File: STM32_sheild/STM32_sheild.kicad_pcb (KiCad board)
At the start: 2 copper layers, 87 x 83.5 mm, 48 parts, among them J1 61612002121503, J2 CN7, J3 CN10, J4 632722100213, J5 691210910002, J6 691210910002, U1 OPA333xxDBV, U2 TPS63031DSK, U3 MCP73831-2-MC, U4 OPA333xxDBV

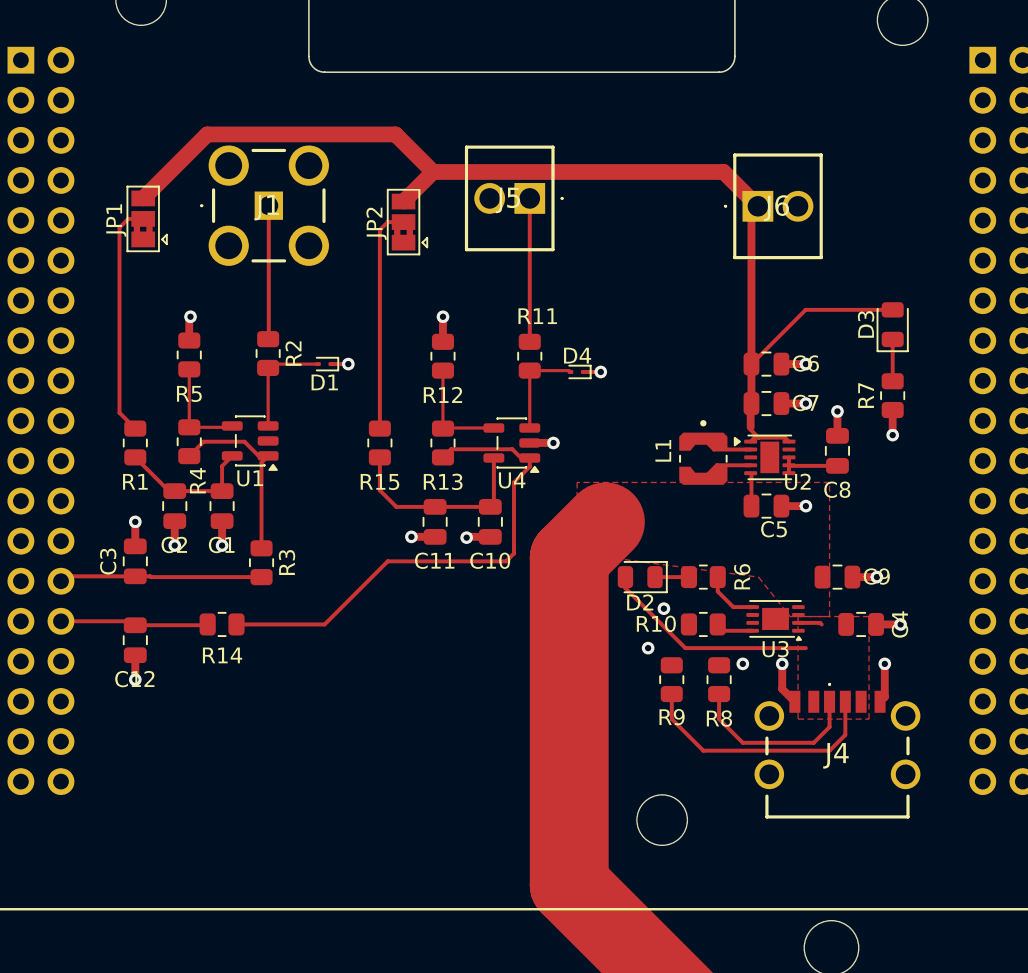
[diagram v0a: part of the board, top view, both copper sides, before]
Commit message: random updates
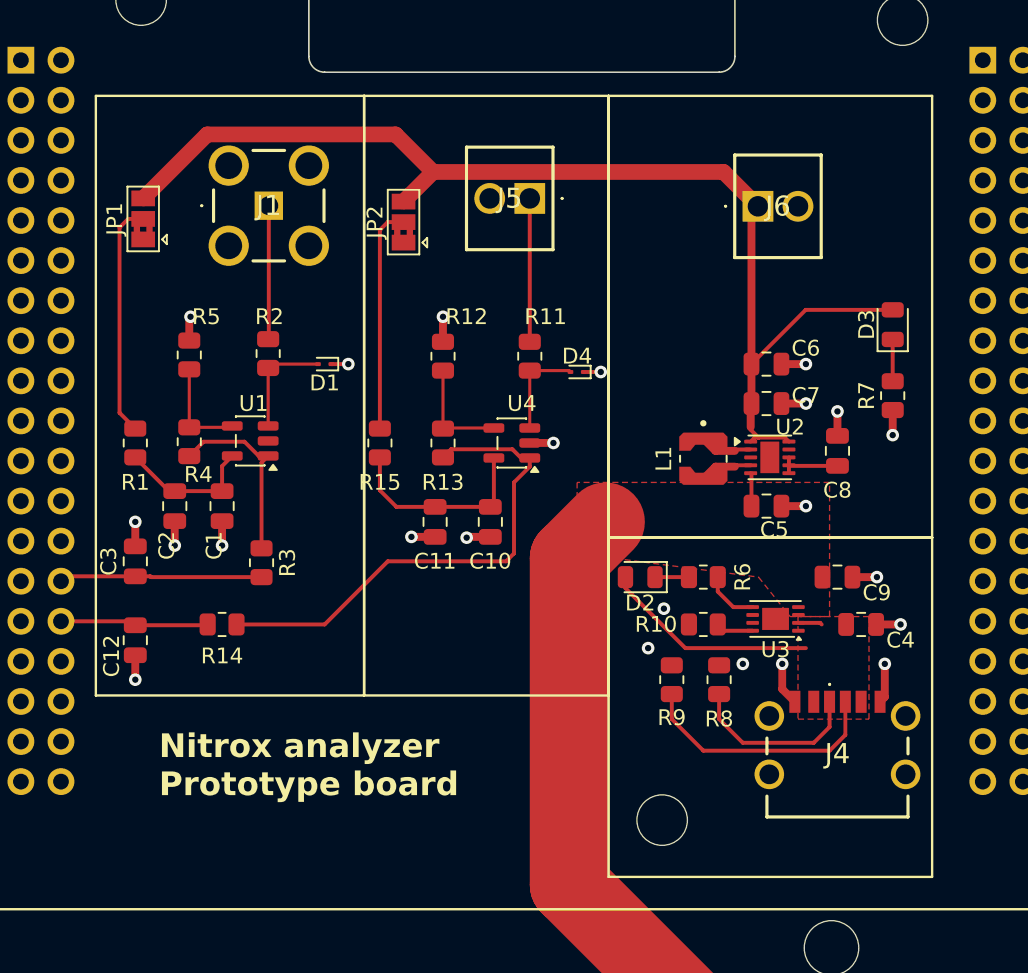
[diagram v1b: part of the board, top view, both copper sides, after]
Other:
- board text added: "Nitrox analyzer Prototype board"
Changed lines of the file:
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@@
 		(tags "resistor")
 		(property "Reference" "R5"
-			(at -2.5 0 180)
+			(at 2.42 1.08 180)
 			(layer "F.SilkS")
 			(effects
@@
 		(tags "WSON NoLead")
 		(property "Reference" "U2"
-			(at 1.7875 1.5875 0)
+			(at 1.2875 -1.9125 0)
 			(layer "F.SilkS")
 			(effects
@@
 		(tags "resistor")
 		(property "Reference" "R2"
-			(at 0 -1.65 90)
+			(at -2.3325 -0.08 180)
 			(layer "F.SilkS")
 			(effects
@@
 		(tags "capacitor")
 		(property "Reference" "C9"
-			(at 2.5 0 180)
+			(at 2.5 1 180)
 			(layer "F.SilkS")
 			(effects
@@
 		)
 		(property "Value" "4.7uF"
-			(at 2 -2 0)
+			(at 0.5 -1.5 0)
 			(layer "F.Fab")
 			(effects
@@
 		(at 148 87.5 -90)
 		(property "Reference" "L1"
-			(at -0.5 2.5 90)
+			(at 0 2.5 270)
 			(layer "F.SilkS")
 			(effects
@@
 		(tags "SOT TO_SOT_SMD")
 		(property "Reference" "U1"
-			(at 0 -2.4 0)
+			(at -0.2175 2.37 0)
 			(layer "F.SilkS")
 			(effects
@@
 		(tags "resistor")
 		(property "Reference" "R12"
-			(at -2.5 0 180)
+			(at 2.5 1.5 180)
 			(layer "F.SilkS")
 			(effects
@@
 		(tags "SOT TO_SOT_SMD")
 		(property "Reference" "U4"
-			(at 0 -2.4 0)
+			(at -0.6375 2.5 0)
 			(layer "F.SilkS")
 			(effects
@@
 		)
 		(property "Value" "OPA333xxDBV"
-			(at -3.1375 2.4 0)
+			(at -4.1375 -2.5 0)
 			(layer "F.Fab")
 			(effects
@@
 		(tags "capacitor")
 		(property "Reference" "C7"
-			(at 2.5 0 0)
+			(at 2.5 -0.5 0)
 			(layer "F.SilkS")
 			(effects
@@
 		)
 		(property "Value" "2.2k"
-			(at -4 0 0)
+			(at -3.5 -1 0)
 			(layer "F.Fab")
 			(effects
@@
 		(tags "capacitor")
 		(property "Reference" "C2"
-			(at 2.5 0 180)
+			(at 2.5 0.5 270)
 			(layer "F.SilkS")
 			(effects
@@
 		)
 		(property "Value" "10uF"
-			(at 0 1.68 90)
+			(at 0.5 1.5 90)
 			(layer "F.Fab")
 			(effects
@@
 		(tags "capacitor")
 		(property "Reference" "C4"
-			(at 2.5 0 90)
+			(at 2.5 1 180)
 			(layer "F.SilkS")
 			(effects
@@
 		(tags "resistor")
 		(property "Reference" "R4"
-			(at 2.5 -0.58 90)
+			(at 2.08 -0.58 180)
 			(layer "F.SilkS")
 			(effects
@@
 		(tags "resistor")
 		(property "Reference" "R11"
-			(at -2.5 -0.5 180)
+			(at -2.5 -1 180)
 			(layer "F.SilkS")
 			(effects
@@
 		(tags "capacitor")
 		(property "Reference" "C12"
-			(at 2.5 0 180)
+			(at 1 1.5 270)
 			(layer "F.SilkS")
 			(effects
@@
 		)
 		(property "Value" "10uF"
-			(at 0 -2.5 90)
+			(at 1 -2 90)
 			(layer "F.Fab")
 			(effects
@@
 		(tags "capacitor")
 		(property "Reference" "C6"
-			(at 2.5 0 180)
+			(at 2.5 -1 180)
 			(layer "F.SilkS")
 			(effects
@@
 		(tags "capacitor")
 		(property "Reference" "C1"
-			(at 2.5 0 180)
+			(at 2.5 0.5 270)
 			(layer "F.SilkS")
 			(effects
@@
 		)
 		(property "Value" "100n"
-			(at 0 -1.5 90)
+			(at 0.5 1.5 90)
 			(layer "F.Fab")
 			(effects
@@
 		)
 	)
+	(gr_rect
+		(start 109.5 64.5)
+		(end 126.5 102.5)
+		(stroke
+			(width 0.15)
+			(type default)
+		)
+		(fill no)
+		(layer "F.SilkS")
+	)
+	(gr_rect
+		(start 126.5 64.5)
+		(end 142 102.5)
+		(stroke
+			(width 0.15)
+			(type default)
+		)
+		(fill no)
+		(layer "F.SilkS")
+	)
+	(gr_rect
+		(start 142 64.5)
+		(end 162.5 92.5)
+		(stroke
+			(width 0.15)
+			(type default)
+		)
+		(fill no)
+		(layer "F.SilkS")
+	)
+	(gr_rect
+		(start 142 92.5)
+		(end 162.5 114)
+		(stroke
+			(width 0.15)
+			(type default)
+		)
+		(fill no)
+		(layer "F.SilkS")
+	)
 	(gr_line
 		(start 84.5 109.5)
@@
 		(layer "Edge.Cuts")
 	)
+	(gr_text "Nitrox analyzer\nPrototype board"
+		(at 113.5 109 0)
+		(layer "F.SilkS")
+		(effects
+			(font
+				(size 1.5 1.5)
+				(thickness 0.3)
+				(bold yes)
+			)
+			(justify left bottom)
+		)
+	)
 	(segment
 		(start 149.3125 98.4)
@@
 	)
 	(segment
-		(start 151 86.9125)
-		(end 148.6825 86.9125)
+		(start 148 86.23)
+		(end 148.77 87)
+		(width 0.5)
+		(layer "F.Cu")
+		(net "Net-(U2-L2)")
+	)
+	(segment
+		(start 148.77 87)
+		(end 150 87)
+		(width 0.5)
+		(layer "F.Cu")
+		(net "Net-(U2-L2)")
+	)
+	(segment
+		(start 150.0875 86.9125)
+		(end 151 86.9125)
 		(width 0.25)
 		(layer "F.Cu")
@@
 	)
 	(segment
-		(start 148.6825 86.9125)
-		(end 148 86.23)
+		(start 150 87)
+		(end 150.0875 86.9125)
 		(width 0.25)
 		(layer "F.Cu")
@@
 	)
 	(segment
-		(start 148.8575 87.9125)
-		(end 148 88.77)
+		(start 148.77 88)
+		(end 150 88)
+		(width 0.5)
+		(layer "F.Cu")
+		(net "Net-(U2-L1)")
+	)
+	(segment
+		(start 150.110666 87.9125)
+		(end 151 87.9125)
+		(width 0.25)
+		(layer "F.Cu")
+		(net "Net-(U2-L1)")
+	)
+	(segment
+		(start 148 88.77)
+		(end 148.77 88)
+		(width 0.5)
+		(layer "F.Cu")
+		(net "Net-(U2-L1)")
+	)
+	(segment
+		(start 150 88)
+		(end 150.023166 88)
 		(width 0.25)
 		(layer "F.Cu")
@@
 	)
 	(segment
-		(start 151 87.9125)
-		(end 148.8575 87.9125)
+		(start 150.023166 88)
+		(end 150.110666 87.9125)
 		(width 0.25)
 		(layer "F.Cu")
